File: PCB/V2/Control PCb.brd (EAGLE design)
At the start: 52.8 x 85.1 mm, 33 parts, among them Q1 DMP2305U-7, Q2 BSS123, Q3 BSS123, U1 V_REG_317DPACK, U2 5ACFEW

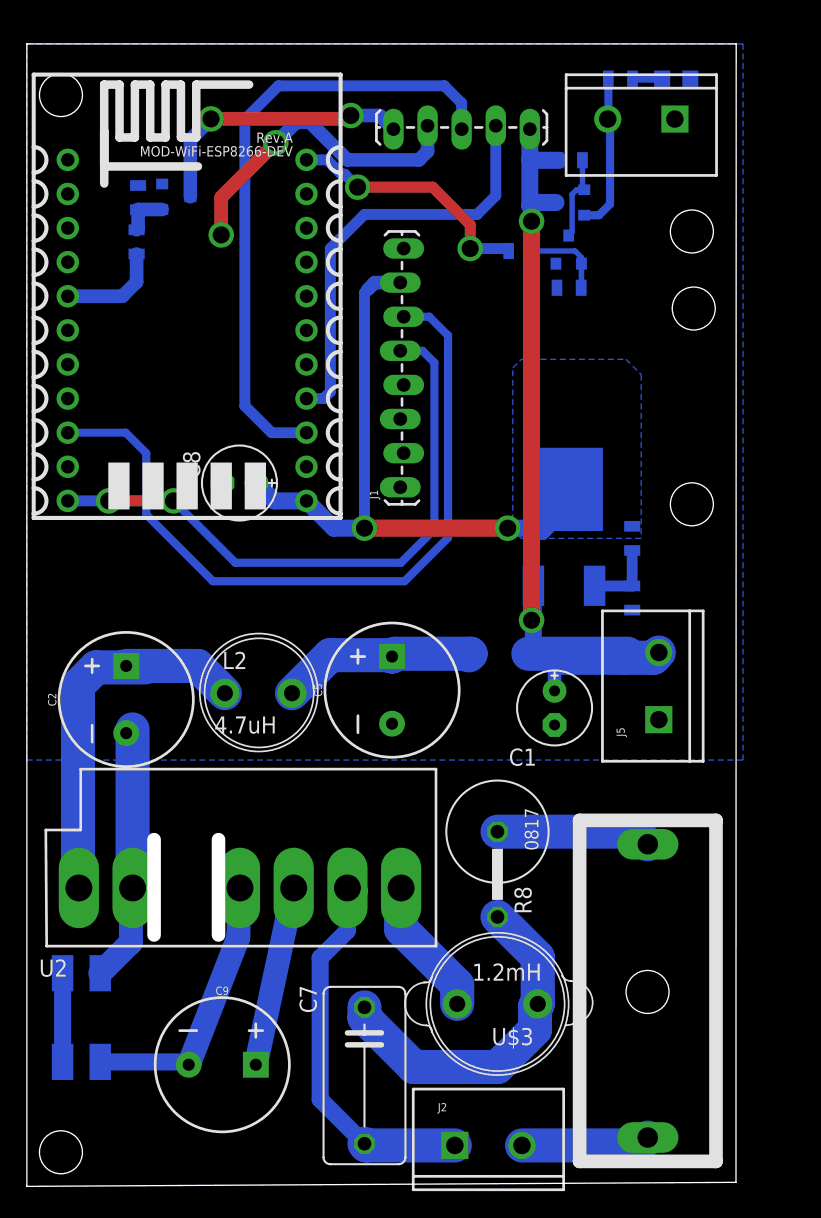
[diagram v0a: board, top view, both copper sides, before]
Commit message: Code + PCB stuff
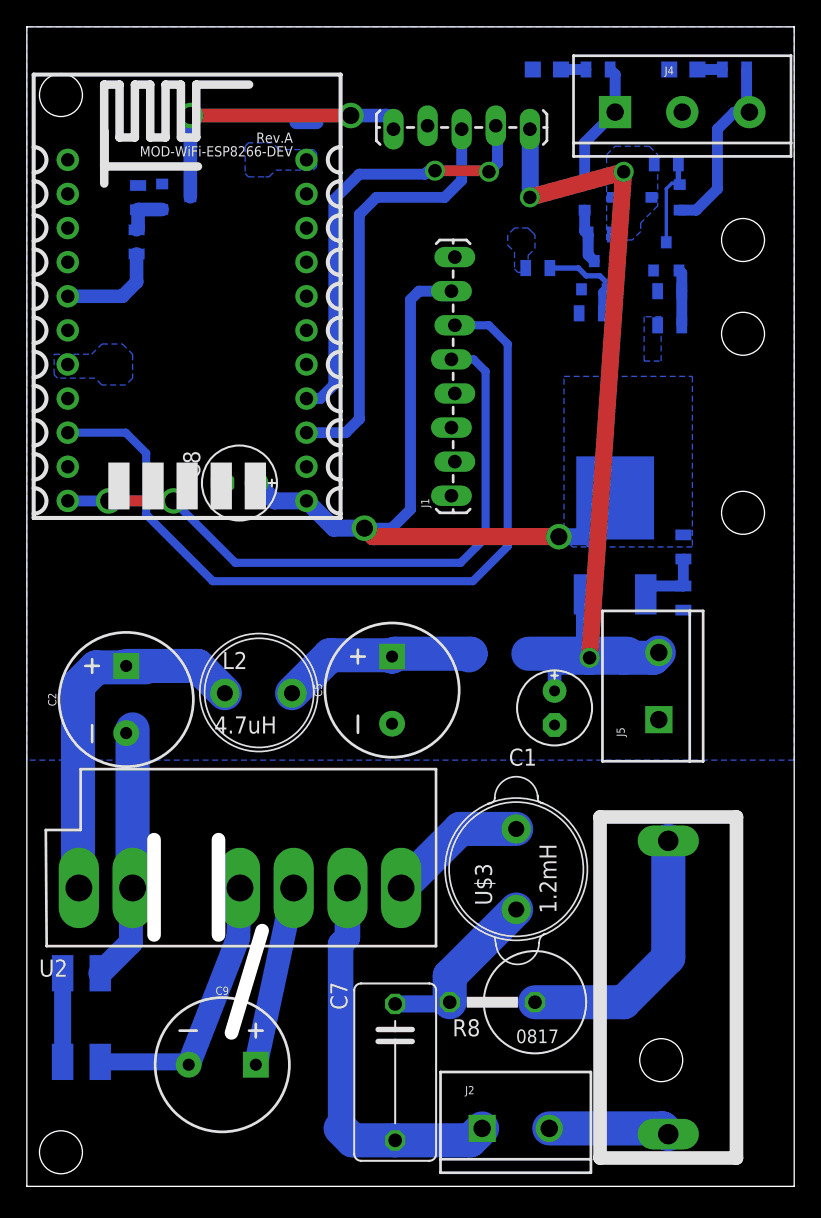
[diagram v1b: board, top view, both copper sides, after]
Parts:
- removed J6: (no value), SparkFun-Connectors:SCREWTERMINAL-5MM-2
- added D3: LED_GREEN, RJC-2:CHIP_LED0805
- added J4: (no value), SparkFun-Connectors:SCREWTERMINAL-5MM-3
- added Q4: DMP2305U-7, RJC-2:SOT23
- added Q5: BSS123, RJC-2:SOT23
- added R11, R12, R13, R5: 0, RJC-2:0805
- moved U$3 10.1 mm to (36.4, 13.5), turned to 90 degrees
- moved D1 9.65 mm to (38.7, 73.0), turned to 270 degrees
- moved R8 7.96 mm to (32.8, 3.56), turned to 180 degrees
- moved R2 5.96 mm to (42.7, 60.7), turned to 180 degrees
- moved R7 3.86 mm to (48.9, 37.5)
- moved J1 3.86 mm to (31.8, 41.3)
- moved U1 3.86 mm to (43.8, 38.7)
- moved R6 3.81 mm to (48.9, 33.7)
- moved Q2 2.69 mm to (42.3, 57.7)
- moved R9 2.52 mm to (42.0, 54.9)
- moved J2 2.40 mm to (33.9, -5.84)
- moved C7 2.30 mm to (27.4, -1.65)
- moved Q1 2.07 mm to (42.5, 63.5), turned to 90 degrees
- moved R3 1.80 mm to (42.5, 73.0), turned to 180 degrees
- moved R1 1.80 mm to (38.1, 58.2)
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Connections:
- new net N$16: J4.3, Q4.2, R5.2
- new net N$19: D3.A, R5.1
- new net N$20: Q4.1, Q5.3, R11.1
- new net N$21: R13.1, U$1.18
- new net N$22: Q5.1, R12.2, R13.2
- net +5V: now also Q4.3, R11.2
- net GND: now also D3.C, J4.2, Q5.2, R12.1; no longer J6.1
- net N$6: now also J4.1; no longer J6.2
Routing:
- net GND: track 43.4 -> 21.1 mm, vias 2 -> 0
- net N$7: track 19.1 -> 0.00 mm, vias 2 -> 0
- net RX: track 46.4 -> 32.1 mm
- net N$16: track 0.00 -> 14.1 mm
- net N$11: track 25.9 -> 13.1 mm
- net +5V: track 63.9 -> 74.9 mm, vias 2 -> 3
- net N$10: track 11.6 -> 20.0 mm
- net N$20: track 0.00 -> 6.68 mm
- net +3V3: track 47.4 -> 53.6 mm
- net SDA: track 55.9 -> 60.7 mm
- net N$22: track 0.00 -> 4.16 mm
- net SCL: track 45.6 -> 49.1 mm
- net N$5: track 6.47 -> 4.09 mm
- net N$6: track 11.7 -> 9.67 mm
- net N$19: track 0.00 -> 1.86 mm
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- added copper zone on layer 16, net +5V
- added copper zone on layer 16, net N$21
- added copper zone on layer 16, net N$7
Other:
- board size 52.8 x 85.1 mm -> 57.1 x 86.4 mm
